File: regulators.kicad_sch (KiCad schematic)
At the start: 62 parts, among them J14 Screw_Terminal_06x01x02, U12 AP64500, U13 AP64500, U14 AP2112K-3.3, U15 TPS7A20xxxDQN

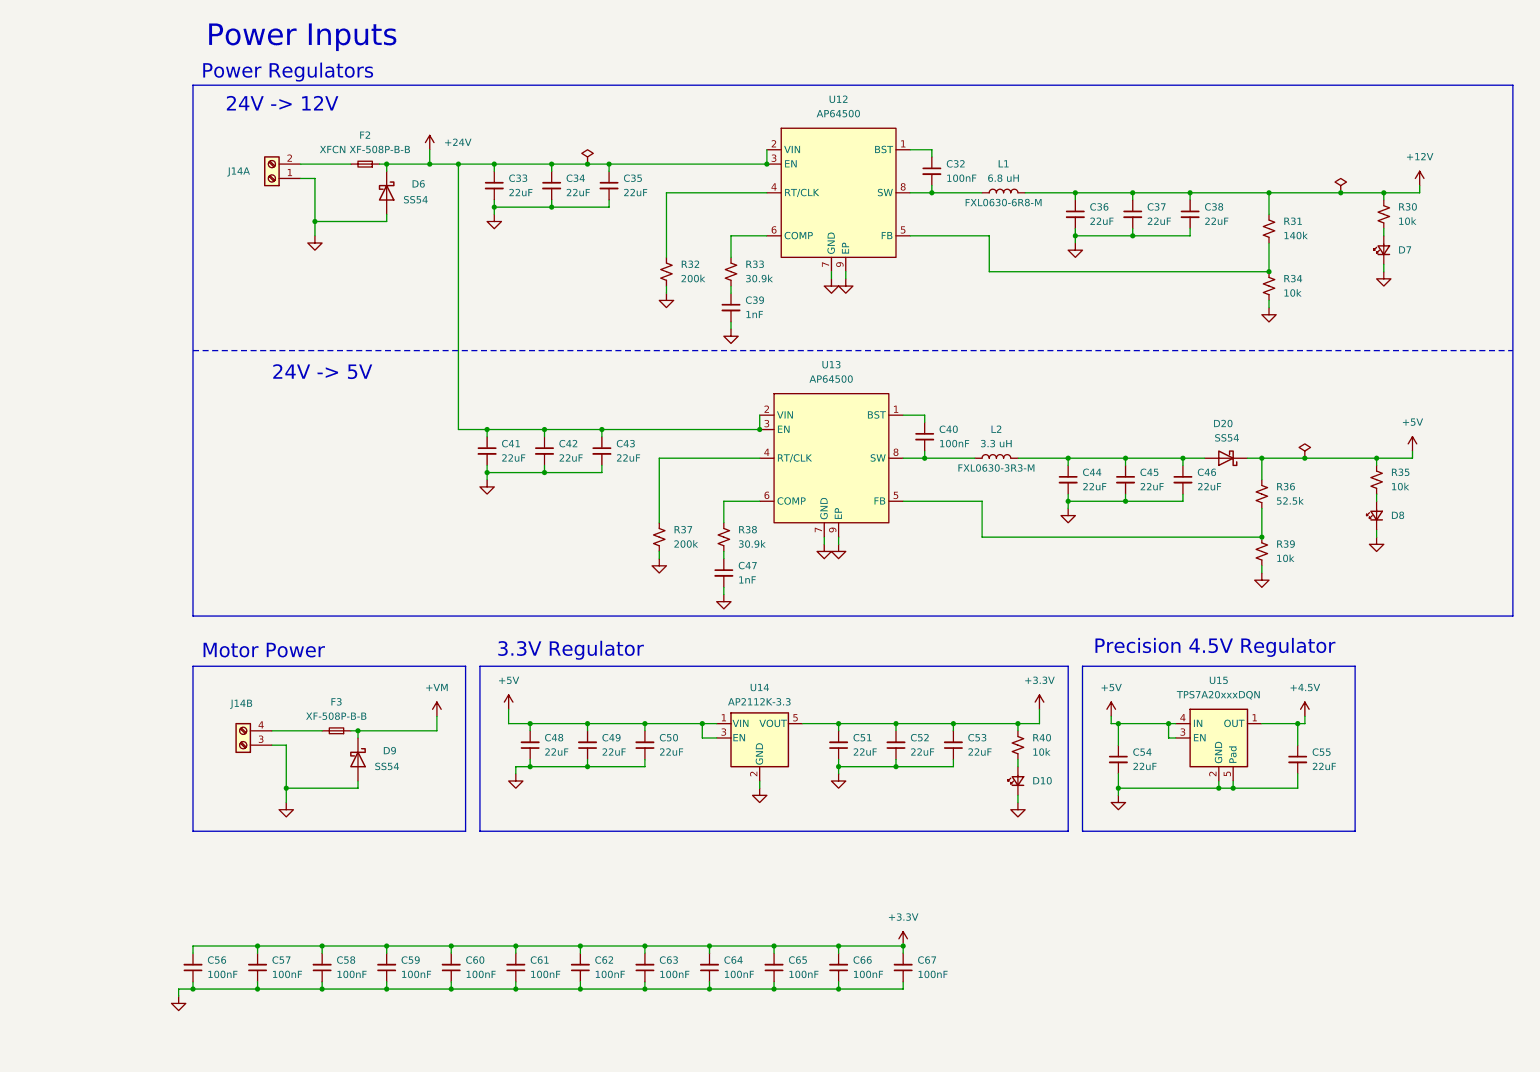
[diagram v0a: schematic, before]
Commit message: a
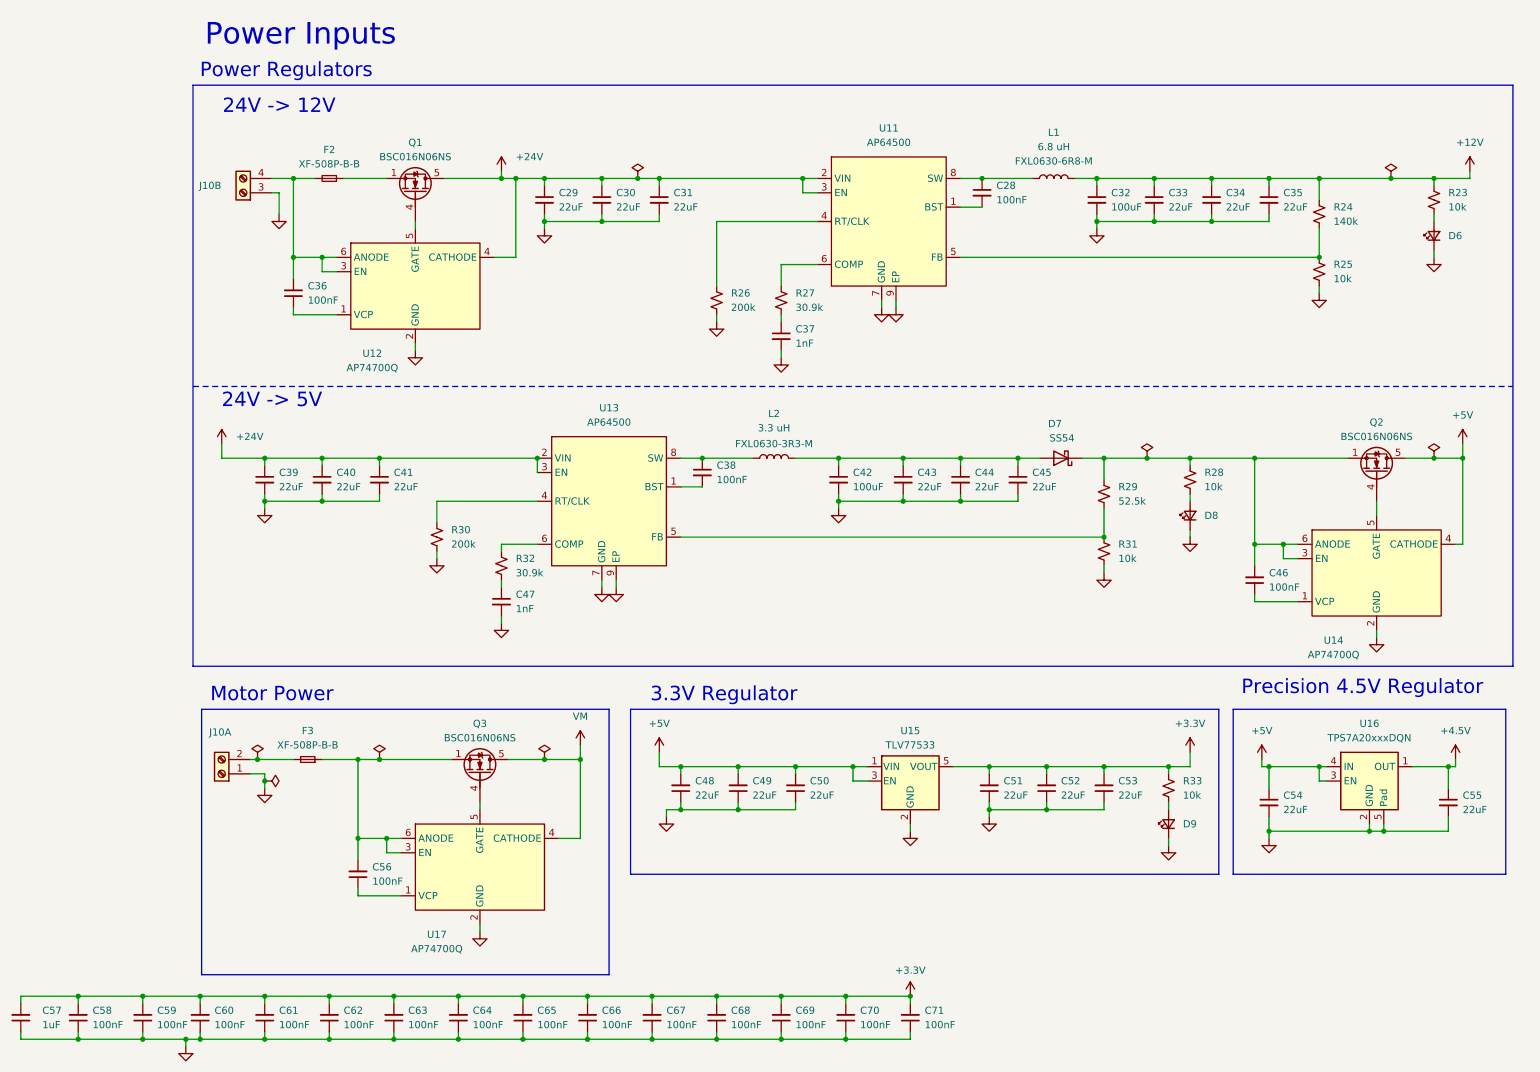
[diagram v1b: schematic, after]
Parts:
- removed D6, D9: SS54, Diode_SMD:D_SMA, symbol Diode:SS38
- removed U12: AP64500, Package_SO:Diodes_SO-8EP, symbol libserie:AP64500-EP
- added C32, C42: 100uF, Capacitor_SMD:CP_Elec_10x10.5, symbol Device:C_Small
- added C36, C46, C56, C58, C59: 100nF, APRLPrints:C_0603, symbol Device:C_Small
- added C57: 1uF, APRLPrints:C_0603, symbol Device:C_Small
- added Q1, Q2, Q3: BSC016N06NS, Package_TO_SOT_SMD:TDSON-8-1, symbol Transistor_FET:CSD18532NQ5B
- added U11: AP64500, libserie:Diodes_SO-8EP, symbol libserie:AP64500-EP
- added U12, U14, U17: AP74700Q, libserie:SOT-6, symbol libserie:AP74700Q
- F2: value XFCN XF-508P-B-B -> XF-508P-B-B
- U13: footprint Package_SO:Diodes_SO-8EP -> libserie:Diodes_SO-8EP
- U15: renamed from U14; value AP2112K-3.3 -> TLV77533
- renumbered C32 to C28, C33 to C29, C34 to C30, C35 to C31, C37 to C33, C38 to C34, C36 to C35, C39 to C37, C40 to C38, C41 to C39, C42 to C40, C43 to C41, C45 to C43, C46 to C44, C44 to C45, C56 to C60, C57 to C61, C58 to C62, C59 to C63, C60 to C64, C61 to C65, C62 to C66, C63 to C67, C64 to C68, C65 to C69, C66 to C70, C67 to C71, D7 to D6, D20 to D7, D10 to D9, J14 to J10, R30 to R23, R31 to R24, R34 to R25, R32 to R26, R33 to R27, R35 to R28, R36 to R29, R37 to R30, R39 to R31, R38 to R32, R40 to R33, U15 to U16
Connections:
- net +12V: now also C32.1
- net +24V: now also Q1.5 (D), U11.2 (VIN), U11.3 (EN), U12.4 (CATHODE); no longer F2.1
- net +3.3V: now also C57.2, C58.2, C59.2
- net +5V: now also Q2.5 (D), U14.4 (CATHODE); no longer D7.1 (K), R28.1, R29.1
- net GND: now also J10.1 (Pin_1), J10.3 (Pin_1), C32.2, C42.2, C57.1, C58.1, C59.1, U11.7 (GND), U11.9 (EP), U12.2 (GND), U14.2 (GND), U17.2 (GND); no longer J10.1 (Pin_1), J10.3 (Pin_1)
- net at L2.1, U13.8 (SW): now also C38.1; no longer C38.2
- net at C43.1, C44.1, C45.1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: now also C42.1
- net at U13.1 (BST): now also C38.2; no longer C38.1
- net at F3.2: now also J10.2 (Pin_2); no longer J10.4 (Pin_2)
- net at R26.1: now also U11.4 (RT/CLK)
- net at R27.1: now also U11.6 (COMP)
- net at F2.2: now also J10.4 (Pin_2), C36.2, U12.3 (EN), U12.6 (ANODE); no longer J10.2 (Pin_2)
- net at R24.2, R25.1: now also U11.5 (FB)
- net at C28.1: now also L1.1, U11.8 (SW)
- net at C28.2: now also U11.1 (BST); no longer L1.1
- net +VM: no longer names the net of F3.1
- net +VM: now also C56.2, Q3.1 (S), Q3.2 (S), Q3.3 (S), U17.3 (EN), U17.6 (ANODE)
- new net: C46.2, D7.1 (K), Q2.1 (S), Q2.2 (S), Q2.3 (S), R28.1, R29.1, U14.3 (EN), U14.6 (ANODE)
- new net: Q2.4 (G), U14.5 (GATE)
- new net: C56.1, U17.1 (VCP)
- new net: F2.1, Q1.1 (S), Q1.2 (S), Q1.3 (S)
- new net: Q1.4 (G), U12.5 (GATE)
- new net: C36.1, U12.1 (VCP)
- new net: C46.1, U14.1 (VCP)
- new net: Q3.4 (G), U17.5 (GATE)
- new net VM: Q3.5 (D), U17.4 (CATHODE)
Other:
- moved on the sheet: C28, C29, C30, C31, C33, C34, C35, C37, C38, C39, C40, C41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
